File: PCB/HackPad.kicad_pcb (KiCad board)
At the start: 2 copper layers, 45 x 65.2 mm, 7 parts, among them SW1 SW_Push, SW2 SW_Push, SW3 SW_Push, SW4 SW_Push, U1 XIAO-RP2040-DIP

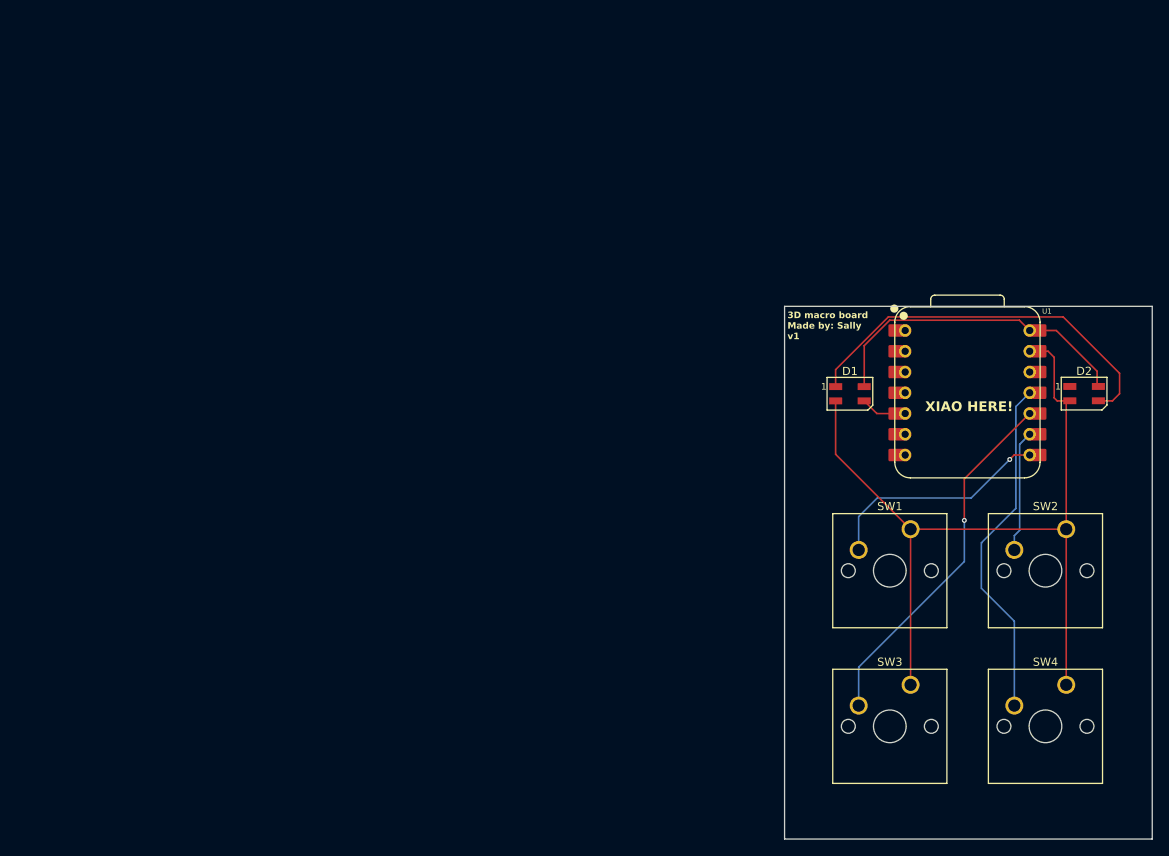
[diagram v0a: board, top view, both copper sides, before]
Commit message: Add files via upload
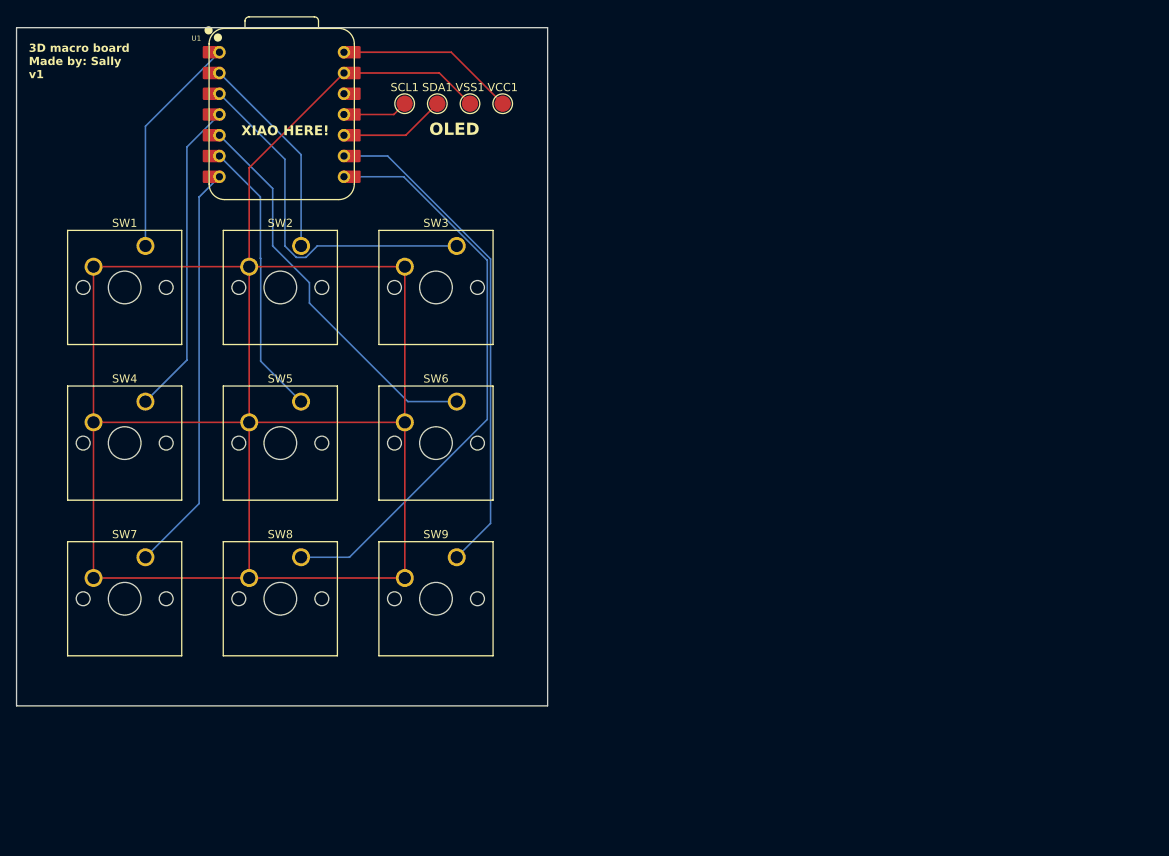
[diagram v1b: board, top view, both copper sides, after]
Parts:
- removed D1, D2: SK6812MINI, LED_SMD:LED_SK6812MINI_PLCC4_3.5x3.5mm_P1.75mm
- added SCL1: TestPoint, TestPoint:TestPoint_Pad_D2.0mm, F.Cu at (133.5, 50.0)
- added SDA1: TestPoint, TestPoint:TestPoint_Pad_D2.0mm, F.Cu at (137.5, 50.0)
- added SW5: SW_Push, Button_Switch_Keyboard:SW_Cherry_MX_1.00u_PCB, F.Cu at (120.8, 86.5)
- added SW6: SW_Push, Button_Switch_Keyboard:SW_Cherry_MX_1.00u_PCB, F.Cu at (139.9, 86.5)
- added SW7: SW_Push, Button_Switch_Keyboard:SW_Cherry_MX_1.00u_PCB, F.Cu at (101.8, 105.5)
- added SW8: SW_Push, Button_Switch_Keyboard:SW_Cherry_MX_1.00u_PCB, F.Cu at (120.8, 105.5)
- added SW9: SW_Push, Button_Switch_Keyboard:SW_Cherry_MX_1.00u_PCB, F.Cu at (139.9, 105.5)
- added VCC1: TestPoint, TestPoint:TestPoint_Pad_D2.0mm, F.Cu at (145.5, 50.0)
- added VSS1: TestPoint, TestPoint:TestPoint_Pad_D2.0mm, F.Cu at (141.5, 50.0)
- moved SW4 117.9 mm to (101.8, 86.5)
- moved SW2 99.9 mm to (120.8, 67.4)
- moved SW1 99.9 mm to (101.8, 67.4)
- moved U1 90.6 mm to (118.5, 51.3)
- moved SW3 77.3 mm to (139.9, 67.4)
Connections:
- SW1 pad 1: GND -> Net-(U1-GPIO26/ADC0/A0)
- SW1 pad 2: Net-(U1-GPIO1/RX) -> GND
- SW2 pad 1: GND -> Net-(U1-GPIO27/ADC1/A1)
- SW2 pad 2: Net-(U1-GPIO2/SCK) -> GND
- SW3 pad 1: GND -> Net-(U1-GPIO28/ADC2/A2)
- SW3 pad 2: Net-(U1-GPIO4/MISO) -> GND
- SW4 pad 1: GND -> Net-(U1-GPIO29/ADC3/A3)
- SW4 pad 2: Net-(U1-GPIO3/MOSI) -> GND
- U1 pad 1: unconnected-(U1-GPIO26/ADC0/A0-Pad1) -> Net-(U1-GPIO26/ADC0/A0)
- U1 pad 2: unconnected-(U1-GPIO27/ADC1/A1-Pad2) -> Net-(U1-GPIO27/ADC1/A1)
- U1 pad 3: unconnected-(U1-GPIO28/ADC2/A2-Pad3) -> Net-(U1-GPIO28/ADC2/A2)
- U1 pad 4: unconnected-(U1-GPIO29/ADC3/A3-Pad4) -> Net-(U1-GPIO29/ADC3/A3)
- U1 pad 6: unconnected-(U1-GPIO7/SCL-Pad6) -> Net-(U1-GPIO7/SCL)
- U1 pad 7: unconnected-(U1-GPIO0/TX-Pad7) -> Net-(U1-GPIO0/TX)
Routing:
- net GND: track 101.8 -> 274.6 mm
- net Net-(U1-GPIO0/TX): track 0.00 -> 50.3 mm
- net Net-(D1-DOUT): track 48.0 -> 0.00 mm
- net Net-(U1-GPIO2/SCK): track 14.9 -> 61.4 mm
- net Net-(U1-GPIO28/ADC2/A2): track 0.00 -> 44.1 mm
- net Net-(U1-GPIO6/SDA): track 4.81 -> 48.1 mm
- net Net-(U1-GPIO1/RX): track 28.1 -> 71.0 mm, vias 1 -> 0
- net Net-(U1-GPIO29/ADC3/A3): track 0.00 -> 38.9 mm
- net Net-(U1-GPIO3/MOSI): track 42.4 -> 7.97 mm
- net Net-(U1-GPIO7/SCL): track 0.00 -> 34.2 mm
- net Net-(U1-GPIO4/MISO): track 44.4 -> 13.0 mm, vias 1 -> 0
- net Net-(U1-GPIO26/ADC0/A0): track 0.00 -> 27.5 mm
- net Net-(U1-GPIO27/ADC1/A1): track 0.00 -> 25.3 mm
- net +5V: track 38.4 -> 22.0 mm
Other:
- board size 45 x 65.2 mm -> 65 x 83 mm
- board text added: "OLED"
